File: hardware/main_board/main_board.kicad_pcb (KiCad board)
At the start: 4 copper layers, 25 x 44 mm, 59 parts, among them J1 FFC_Prog_Conn, Q1 TP0610T, U1 BT840F, U2 LP5813

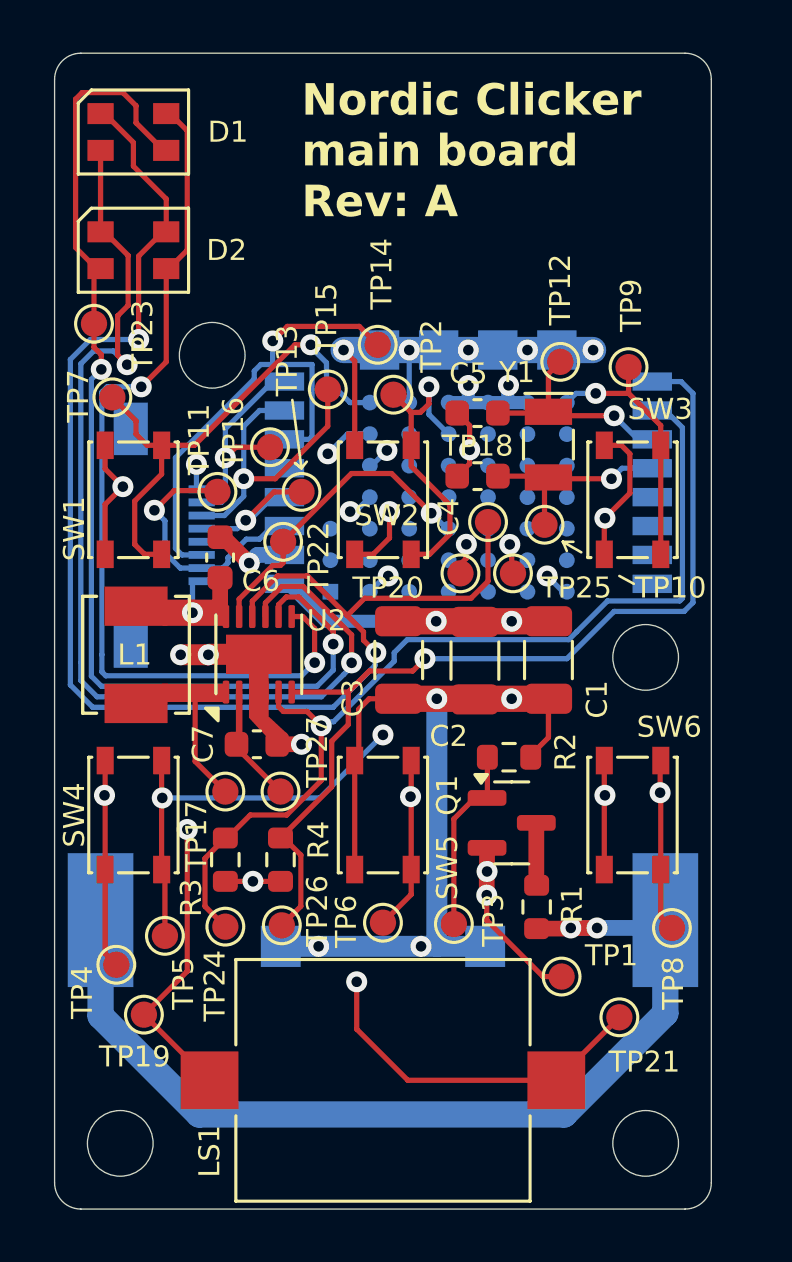
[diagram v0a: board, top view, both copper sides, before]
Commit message: Rev. A finished
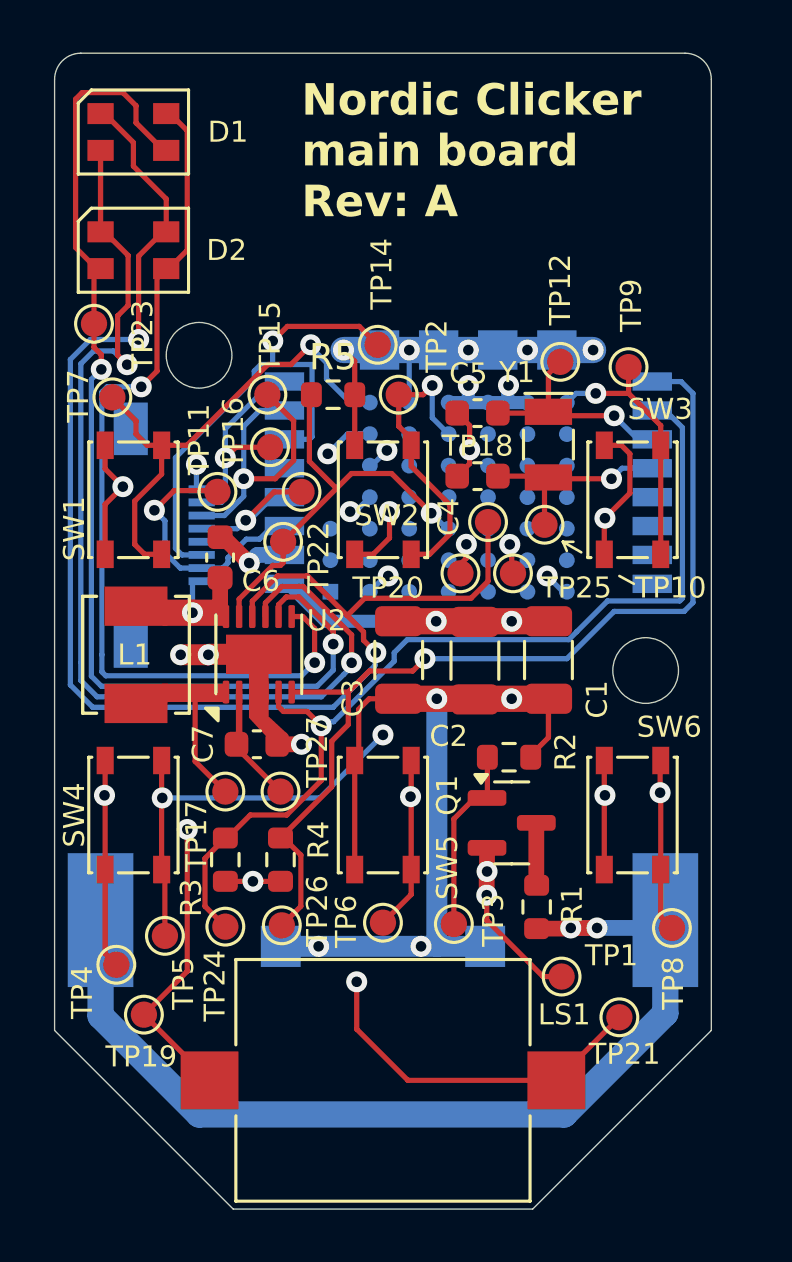
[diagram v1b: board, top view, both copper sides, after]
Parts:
- removed H3, H4: MountingHole, KiPLM_Footprints:Hole_2.5mm_Keepout_4mm
- added R5: 1MΩ, Resistor_SMD:R_0603_1608Metric, F.Cu at (110.6, 113.0)
- C1, C2, C3: value ~ -> 100uF
- C4, C5: value ~ -> 8pF
- C6, C7: value ~ -> 22uF
- L1: value ~ -> 1uH
- R1: value Resistor -> 22Ω
- R2, R3, R4: value Resistor -> 10kΩ
- SW1, SW2, SW3, SW4, SW5, SW6: value ~ -> PTS810SJG250SMTR LFS
- TP1, TP10, TP11, TP12, TP13, TP14, TP15, TP16, TP17, TP18, TP19, TP2, TP20, TP21, TP22, TP23, TP24, TP25, TP26, TP27, TP3, TP4, TP5, TP6, TP7, TP8, TP9: value ~ -> Test_Point
- Y1: value ~ -> 32.768kHz
- moved TP15 2.31 mm to (108.1, 113.0)
- moved H1 0.50 mm to (105.5, 111.5)
- moved H2 0.50 mm to (122.5, 123.5)
- moved TP2 0.20 mm to (113.1, 113.0)
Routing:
- net EN: track 12.0 -> 16.0 mm
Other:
- outline, holes or cut-outs redrawn
